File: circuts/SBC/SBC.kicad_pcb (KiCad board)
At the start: 2 copper layers, 367 parts, among them IC1 PIC16F15243-I_SS, J1 640456-3, J10 DE9_Plug, J11 buzzer, J13 Conn_01x04_Pin, J14 5v Power, J15 Barrel_Jack_MountingPin, J2 B5B-XH-A_LF__SN_, J3 Power, J4 DE9_Plug, J5 OSTTC060162, J6 XT60-M, J7 OSTTC060162, J8 DE9_Plug, J9 Conn_02x04_Odd_Even, Q1 MMBTA06, Q10 BC817, Q11 AO3400A, Q2 MMBTA06, Q3 MMBTA06, Q4 IRFS4227, Q5 MMBTA06, Q6 MMBTA06, Q7 MMBTA06, Q8 IRFS4227, SW1 SW_Push, SW2 SW_Push, SW3 SW_Push, SW4 SW_Push, SW5 SW_Push, SW6 rst, SW7 SW_Push, U1 UC3843, U10 ESP32-DEVKIT-V1, U12 L7805, U13 L7805, U14 L7809, U2 BTS7960B, U3 BTS7960B, U4 LM358DT, U5 AMS1117-3.3, U7 BTS7960B, U8 BTS7960B, U9 LM358DT

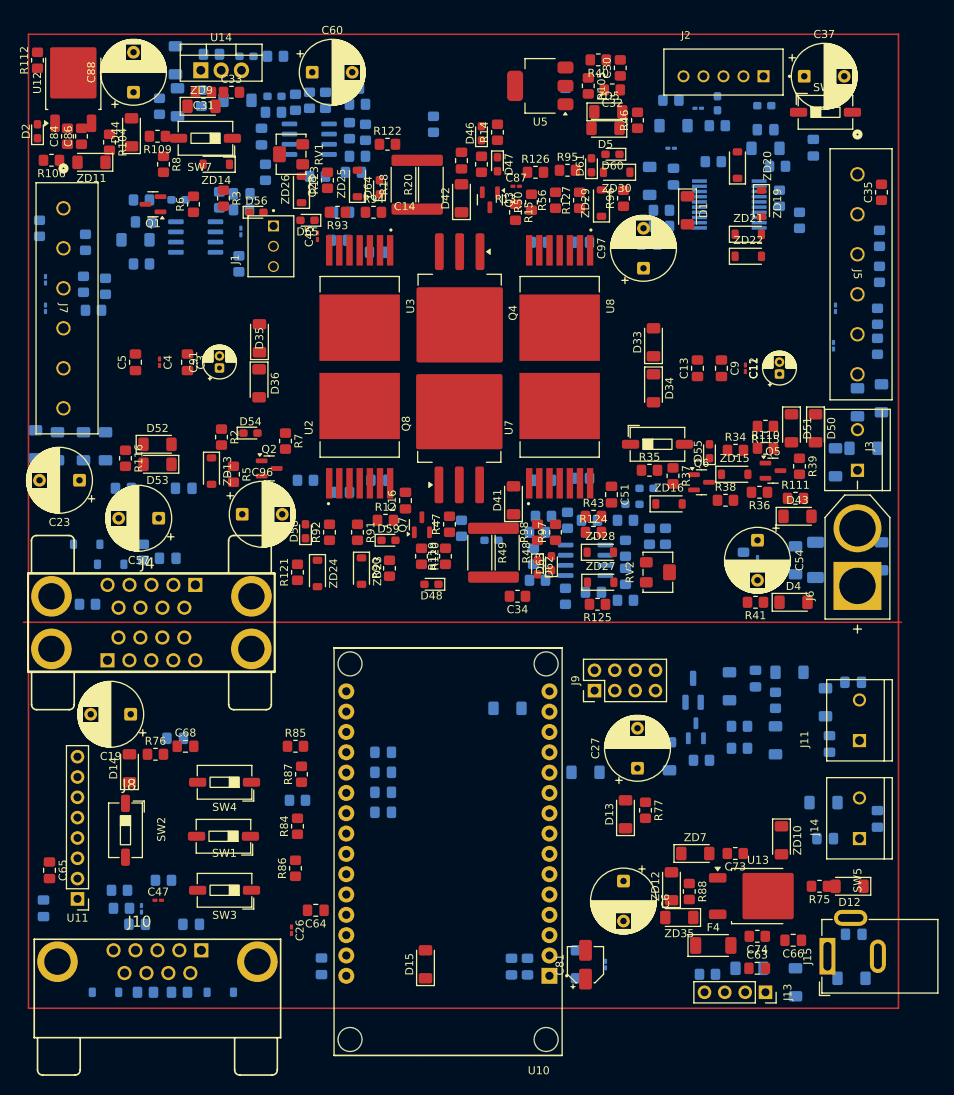
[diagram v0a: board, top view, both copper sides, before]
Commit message: siddyq at fanaly
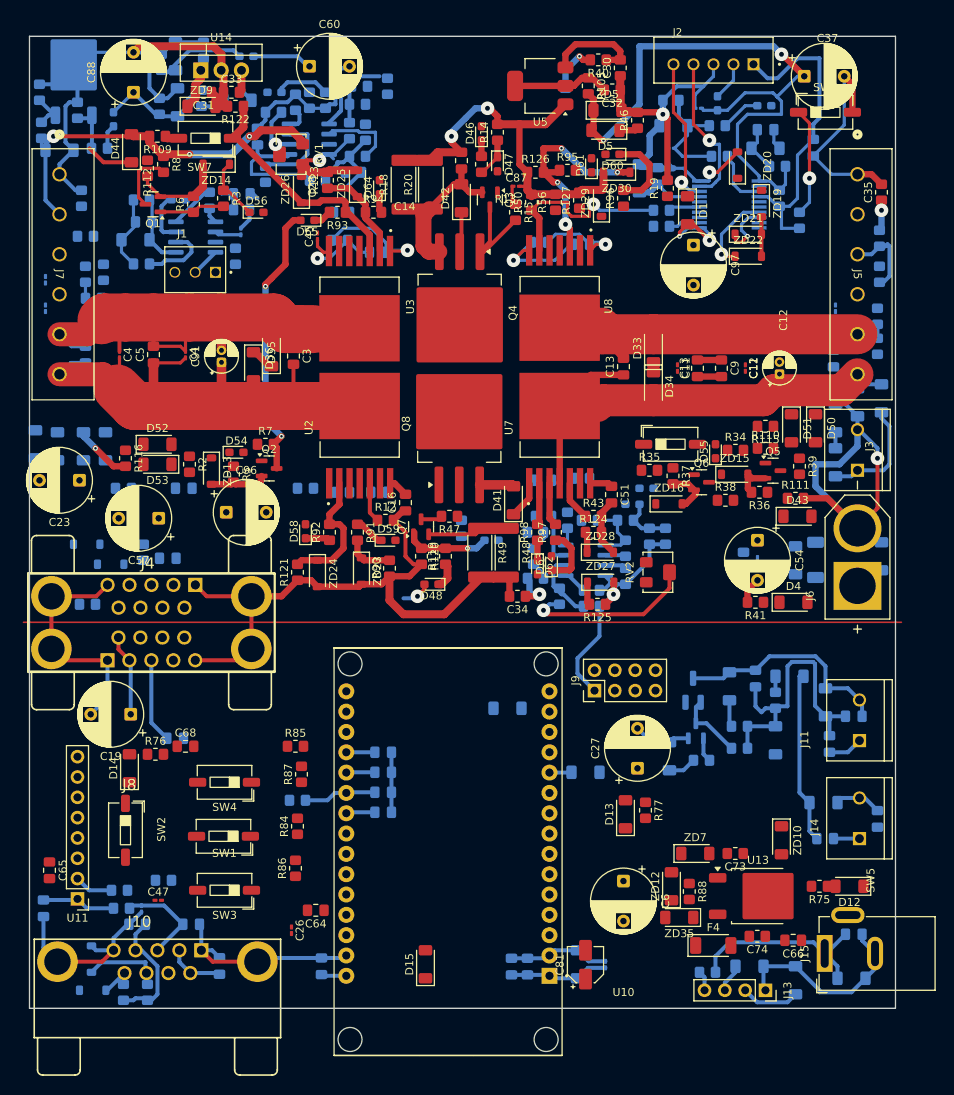
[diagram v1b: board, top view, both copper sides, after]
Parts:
- added C11: 1nf, Capacitor_SMD:C_0201_0603Metric_Pad0.64x0.40mm_HandSolder, F.Cu at (243.5, 80.0)
- added C13: 2uf, Capacitor_SMD:C_0805_2012Metric_Pad1.18x1.45mm_HandSolder, F.Cu at (236.8, 79.8)
- added C4: 1nf, Capacitor_SMD:C_0201_0603Metric_Pad0.64x0.40mm_HandSolder, F.Cu at (173.8, 78.3)
- added C5: 2uf, Capacitor_SMD:C_0805_2012Metric_Pad1.18x1.45mm_HandSolder, B.Cu at (169.5, 78.3)
- added C9: 100nf, Capacitor_SMD:C_0805_2012Metric_Pad1.18x1.45mm_HandSolder, B.Cu at (263.0, 78.8)
- C63, C84, C86, D2, R104, R106, U12, ZD11: moved to B.Cu
- R19: moved to F.Cu
- moved C63 67.2 mm to (186.2, 154.7), turned to 90 degrees
- moved R122 19.6 mm to (188.2, 47.2), turned to 180 degrees
- moved R112 19.3 mm to (177.2, 55.0), turned to -90 degrees
- moved ZD33 16.6 mm to (170.2, 153.8), turned to 90 degrees
- moved C3 13.3 mm to (195.5, 78.5)
- moved D2 9.62 mm to (173.0, 48.9)
- moved J1 9.28 mm to (185.8, 68.0), turned to 0 degrees
- moved R42 9.03 mm to (184.2, 40.2), turned to 90 degrees
- moved R104 8.63 mm to (164.0, 50.2)
- moved C86 7.60 mm to (163.8, 45.5), turned to -90 degrees
- moved R25 7.46 mm to (207.2, 44.8), turned to 90 degrees
- moved R19 7.35 mm to (242.2, 57.5), turned to 90 degrees
- moved C97 6.89 mm to (245.5, 64.6), turned to -90 degrees
- moved C24 6.45 mm to (169.0, 58.8)
- moved R100 6.33 mm to (179.0, 41.8), turned to -90 degrees
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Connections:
- C24 pad 1: 3.3V -> 3.3v
- C35 pad 1: 3.3V -> 3.3v
- C36 pad 1: 3.3V -> 3.3v
- C37 pad 1: 3.3V -> 3.3v
- C38 pad 2: 3.3V -> 3.3v
- C47 pad 1: 3.3V -> 3.3v
- C50 pad 1: 3.3V -> 3.3v
- C53 pad 1: 3.3V -> 3.3v
- C68 pad 1: 3.3V -> 3.3v
- D6 pad 1: 3.3V -> 3.3v
- IC1 pad 1: 3.3V -> 3.3v
- J10 pad 4: 3.3V -> 3.3v
- J4 pad 4: 3.3V -> 3.3v
- J8 pad 4: 3.3V -> 3.3v
- J9 pad 2: 3.3V -> 3.3v
- R101 pad 1: 3.3V -> 3.3v
- R105 pad 2: 3.3V -> 3.3v
- R107 pad 2: 3.3V -> 3.3v
- R113 pad 1: 3.3V -> 3.3v
- R64 pad 1: 3.3V -> 3.3v
- R65 pad 2: 3.3V -> 3.3v
- R66 pad 1: 3.3V -> Net-(R66-Pad1)
- R67 pad 1: 3.3V -> 3.3v
- R68 pad 1: 3.3V -> Net-(R66-Pad1)
- R69 pad 2: 3.3V -> 3.3v
- R70 pad 2: 3.3V -> 3.3v
- R71 pad 2: 3.3V -> 3.3v
- R76 pad 2: 3.3V -> 3.3v
- R80 pad 2: 3.3V -> 3.3v
- ZD5 pad 1: 3.3V -> 3.3v
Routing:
- net GND: track 0.00 -> 594.0 mm, vias 0 -> 10
- net 5v+: track 0.00 -> 103.5 mm, vias 0 -> 4
- net 3.3v: track 0.00 -> 100.3 mm, vias 0 -> 5
- net HV: track 0.00 -> 94.7 mm, vias 0 -> 2
- net M2_R: track 0.00 -> 72.9 mm, vias 0 -> 1
- net M2_L: track 0.00 -> 62.3 mm
- net M1_R: track 0.00 -> 59.6 mm
- net M1_L: track 0.00 -> 47.1 mm
- net Mcler: track 0.00 -> 39.5 mm
- net tst1: track 0.00 -> 36.9 mm, vias 0 -> 5
- net buzzing_vcc: track 0.00 -> 36.5 mm
- net tst2: track 0.00 -> 35.8 mm
- net INH2: track 0.00 -> 34.8 mm, vias 0 -> 2
- net buzzing_gnd: track 0.00 -> 28.0 mm
- net Net-(R22-Pad2): track 0.00 -> 27.4 mm
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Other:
- board outline added: 108.2 x 121.5 mm
- board text added: "1N4004-T_NRND"
- board text added: "C12"
